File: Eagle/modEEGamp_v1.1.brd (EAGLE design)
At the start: 111.4 x 64.8 mm, 131 parts, among them IC2 INA217P, IC204 TLC277P, IC3 TLC277P, IC4 INA217P, IC5 TLC277P, P1 20k, P203 20k, Q1 BC547, Q2 BC557, Q202 BC557, Q204 BC557, Q206 BC547, Q208 BC547, Q3 BC547, Q4 BC557

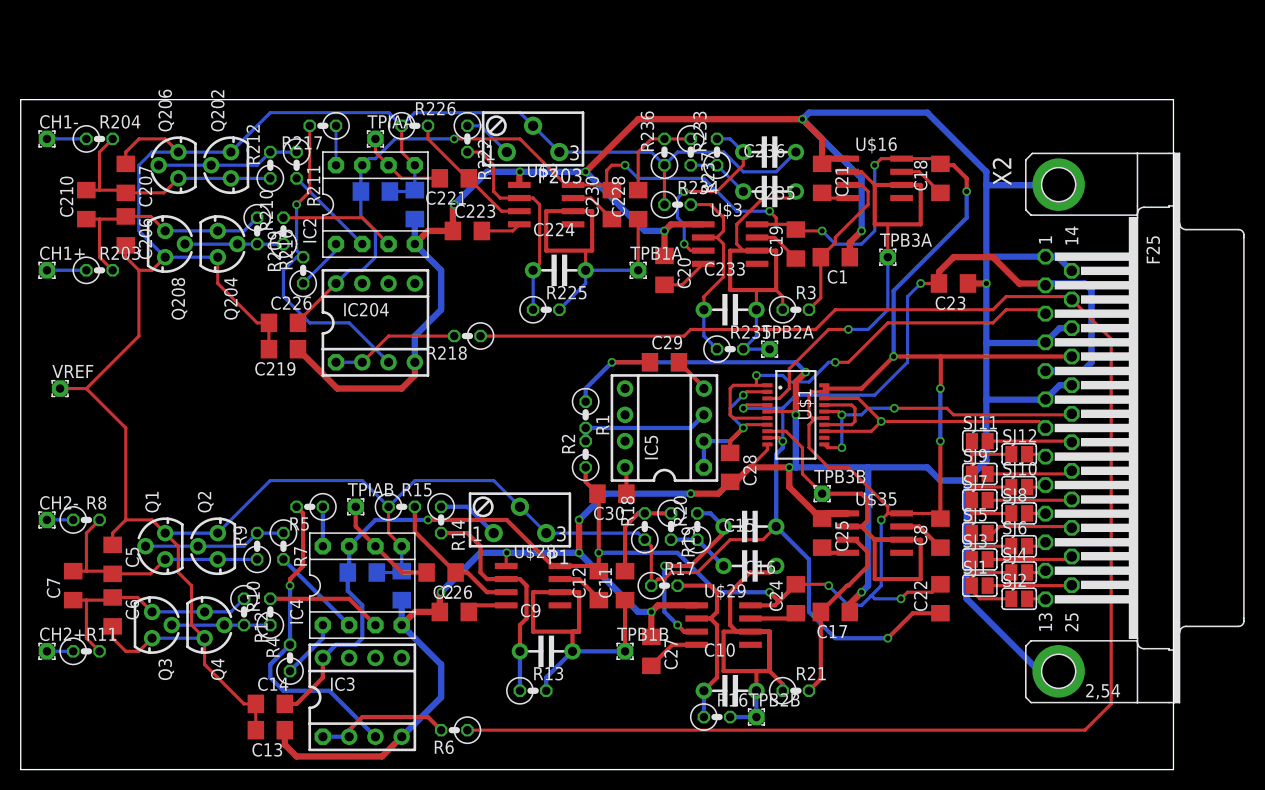
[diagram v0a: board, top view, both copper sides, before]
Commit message: Finished up chanes to DB25
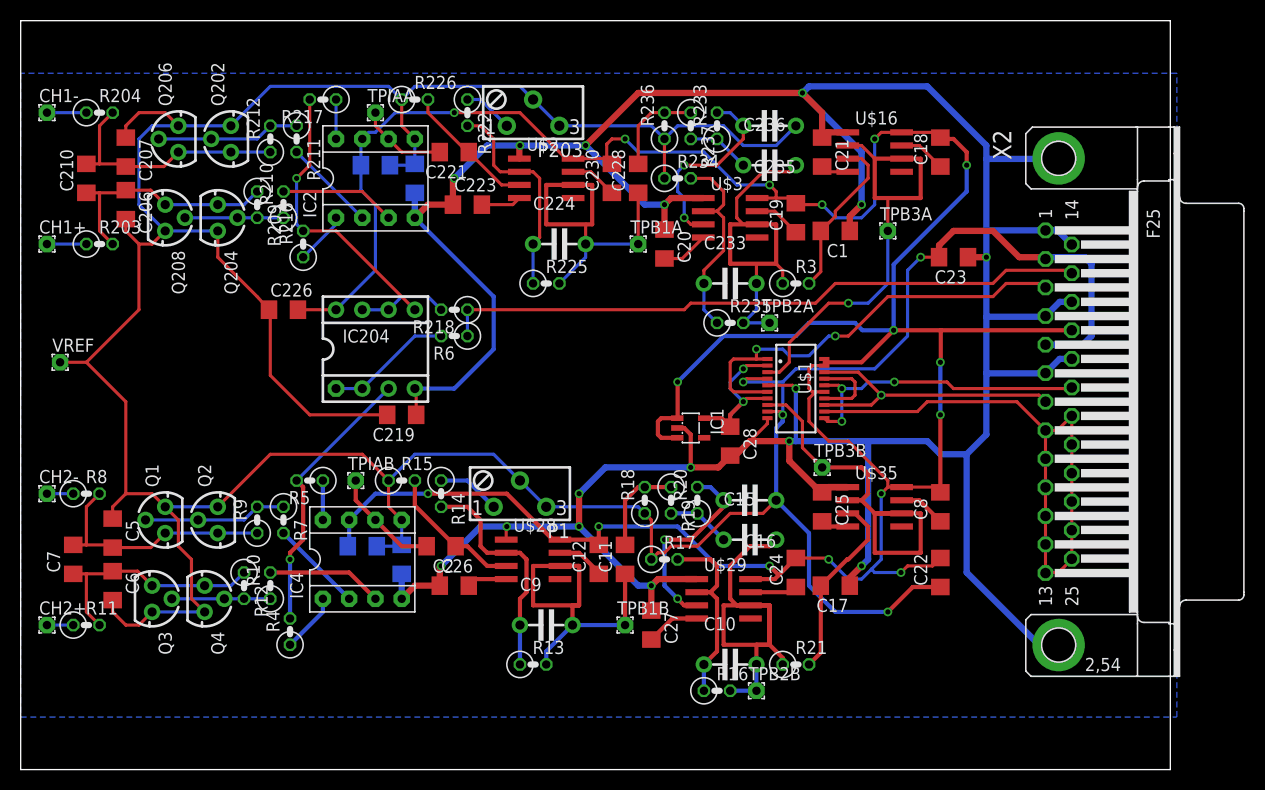
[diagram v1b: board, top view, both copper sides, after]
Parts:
- removed C13, C14, C29, C30: 100nF, resistor:C1206
- removed IC3, IC5: TLC277P, BURR:DIL-08
- removed R1, R2: 10k, resistor:0207/2V
- removed SJ1, SJ10, SJ11, SJ12, SJ2, SJ3, SJ4, SJ5, SJ6, SJ7, SJ8, SJ9: (no value), jumper:SJ
- added IC1: (no value), v-reg-micrel:SOT23-5
- moved R6 38.1 mm to (41.9, 41.9)
- moved C219 13.1 mm to (36.8, 34.3)
- moved R218 2.84 mm to (41.9, 44.5)
- moved C19 2.54 mm to (74.9, 53.3)
- moved Q204 2.54 mm to (19.1, 53.3)
- moved Q208 2.54 mm to (14.0, 53.3)
- moved U$3 2.54 mm to (68.6, 53.3)
- moved C15 2.54 mm to (70.5, 22.2)
- moved CH2- 2.54 mm to (2.54, 26.7)
- moved P1 2.54 mm to (48.3, 26.7)
- moved R14 2.54 mm to (40.6, 26.7)
- moved R15 2.54 mm to (36.8, 27.9)
- moved R5 2.54 mm to (27.9, 27.9)
- moved R8 2.54 mm to (6.35, 26.7)
- moved TPIAB 2.54 mm to (32.4, 27.9)
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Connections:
- removed net N$68: C30.1, IC5.8
- removed net N$69: SJ1.2, X2.25
- removed net N$70: SJ2.2, X2.13
- removed net N$71: SJ3.2, X2.24
- removed net N$72: SJ4.2, X2.12
- removed net N$73: SJ5.2, X2.23
- removed net N$74: SJ6.2, X2.11
- removed net N$75: SJ7.2, X2.22
- removed net N$76: SJ8.2, X2.10
- removed net N$77: SJ12.2, X2.8
- removed net N$78: SJ11.2, X2.20
- removed net N$79: SJ9.2, X2.21
- removed net N$80: SJ10.2, X2.9
- removed net N$81: SJ1.1, SJ10.1, SJ11.1, SJ12.1, SJ2.1, SJ3.1, SJ4.1, SJ5.1, SJ6.1, SJ7.1, SJ8.1, SJ9.1
- removed net N$9: IC5.3, R1.2, R2.2
- net +5V/2: now also IC1.1, IC1.3; no longer C14.2, C30.2, IC3.8, R2.1
- net AGND: now also IC1.2; no longer C13.1, C29.1, IC3.4, R1.1
- net N$12: now also IC204.5; no longer IC204.3
- net N$13: now also IC204.3; no longer IC3.3
- net N$2: now also IC1.5; no longer IC5.1, IC5.2
- net N$3: now also U$1.12, X2.10, X2.11, X2.12, X2.13, X2.20, X2.21, X2.22, X2.23, X2.24, X2.25, X2.8, X2.9; no longer C29.2, IC5.4
- net N$35: now also IC204.1, IC204.2; no longer IC3.1, IC3.2
- net N$52: now also IC204.6, IC204.7; no longer IC204.1, IC204.2
- net VCOM: no longer C13.2, C14.1
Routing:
- net N$66: track 162.8 -> 62.7 mm
- net AGND: track 403.4 -> 347.4 mm, vias 18 -> 16
- net N$3: track 3.54 -> 56.7 mm
- net N$81: track 37.7 -> 0.00 mm
- net N$9: track 13.2 -> 0.00 mm
- net N$73: track 8.44 -> 0.00 mm
- net N$79: track 8.25 -> 0.00 mm
- net N$71: track 8.24 -> 0.00 mm
- net N$78: track 8.17 -> 0.00 mm
- net N$75: track 8.16 -> 0.00 mm
- net N$69: track 8.15 -> 0.00 mm
- net +5V/2: track 290.3 -> 298.3 mm, vias 15 -> 16
- net VCOM: track 374.5 -> 380.2 mm
- net N$13: track 30.6 -> 26.7 mm
- net N$52: track 12.5 -> 8.67 mm
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- added copper zone on layer 16, net AGND
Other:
- board size 111.4 x 64.8 mm -> 111.1 x 72.4 mm
